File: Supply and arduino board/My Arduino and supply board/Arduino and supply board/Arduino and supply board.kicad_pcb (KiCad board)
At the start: 2 copper layers, 68.6 x 53.3 mm, 75 parts, among them IC1 MC33269ST-5.0T3-Arduino_and_s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, IC2 MC33269D-5.0-Arduino_and_supp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, Q1 16MHz, Q2 16MHz, T1 FDN340V, U1 LP2985-3.3, U1A1 LM358D, U1B1 LM358D, U1C1 LM358D, X1 USB_B, Y1 16MHz, Y2 16MHz

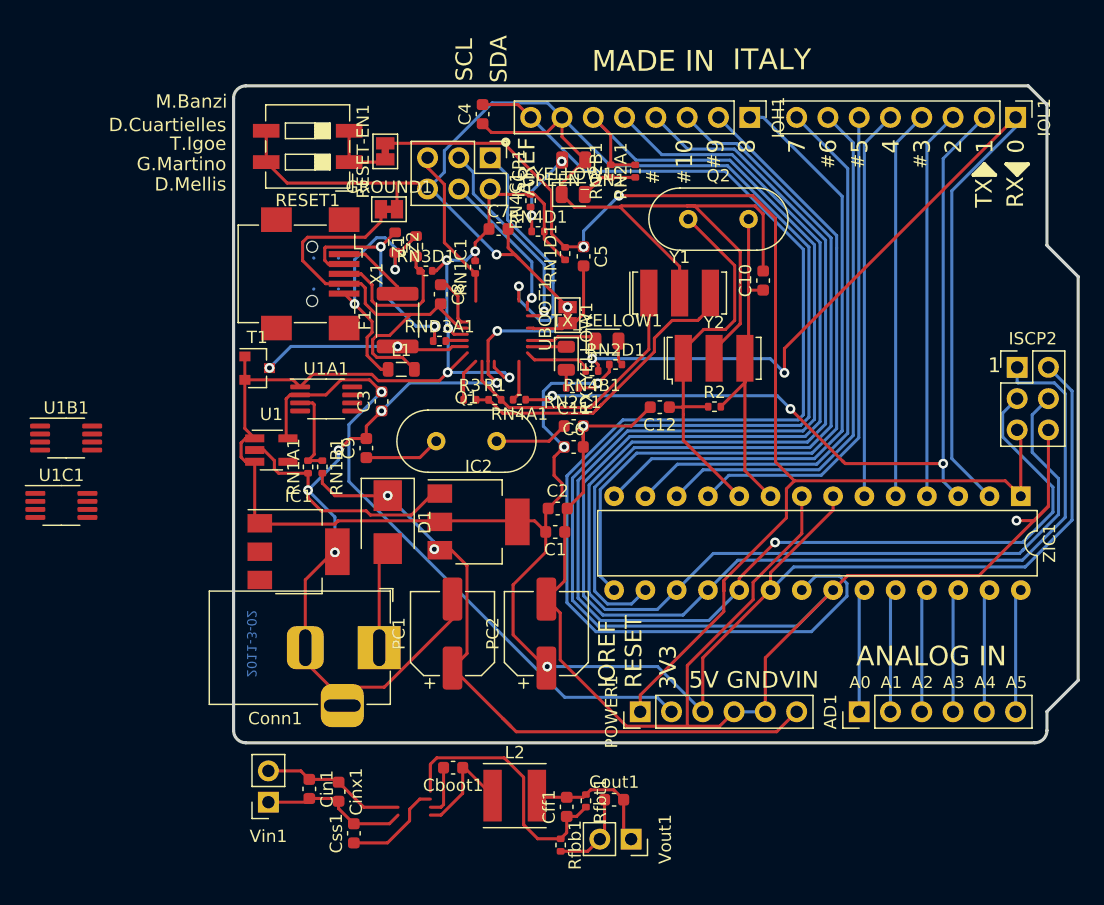
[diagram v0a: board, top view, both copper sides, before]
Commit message: new work on board
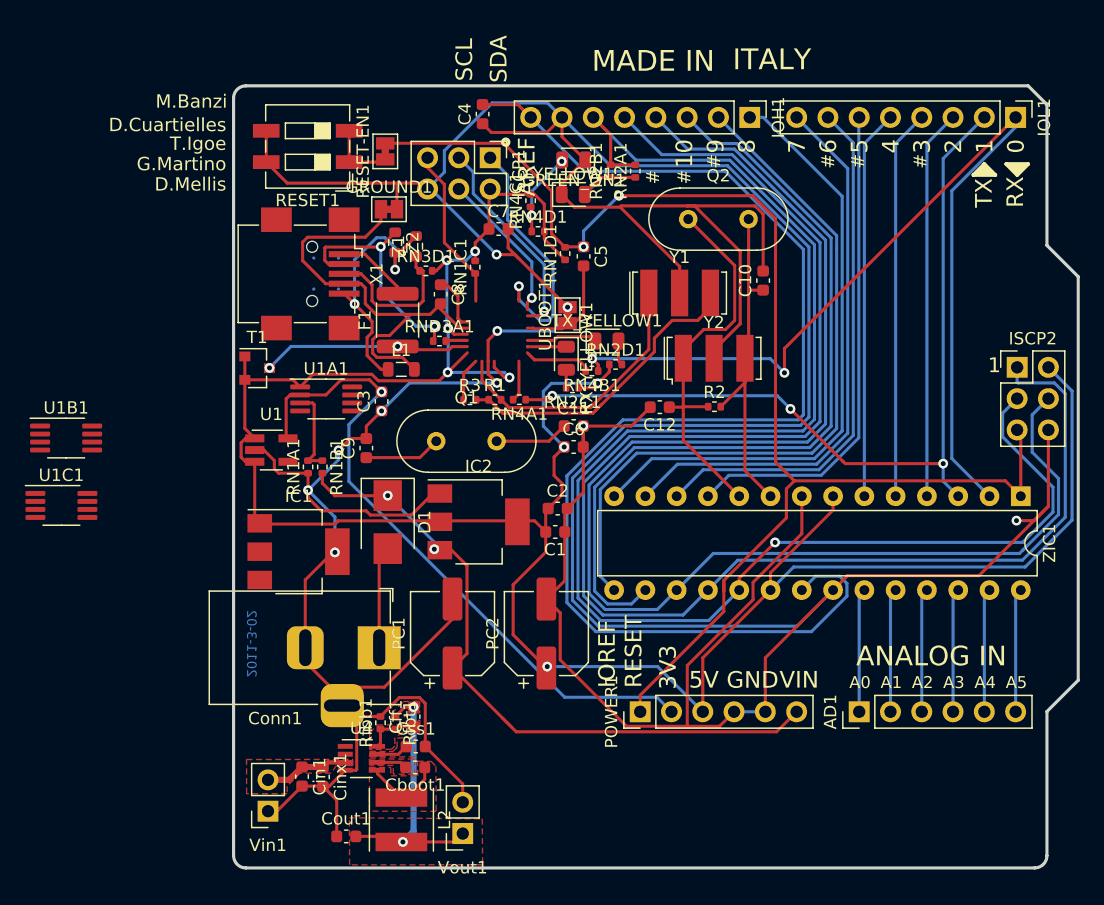
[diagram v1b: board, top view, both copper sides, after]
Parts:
- added U4: Arduino_and_supply_board-cache_Arduino_and_supply_board-cac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, Package_TO_SOT_SMD:TSOT-23-8, F.Cu at (142.6, 100.9)
- moved Cout1 22.0 mm to (141.4, 107.3)
- moved Rfbb1 17.7 mm to (144.1, 98.0), turned to 90 degrees
- moved Rfbt1 16.7 mm to (145.3, 98.1)
- moved Cff1 14.4 mm to (146.8, 97.6)
- moved Vout1 13.7 mm to (150.8, 107.0), turned to 180 degrees
- moved L2 9.41 mm to (145.8, 105.9), turned to 270 degrees
- moved Css1 8.65 mm to (147.0, 100.0), turned to 0 degrees
- moved Cboot1 3.08 mm to (147.0, 101.7)
- moved Cinx1 1.75 mm to (139.5, 102.4)
- moved Cin1 1.17 mm to (137.8, 102.4)
- moved Vin1 0.73 mm to (135.0, 105.2)
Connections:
- Cboot1 pad 2: (no net) -> Net-(Cboot1-Pad2)
- Css1 pad 1: (no net) -> Net-(Css1-Pad1)
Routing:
- net (no net): track 0.09 -> 77.8 mm, vias 0 -> 3
- net /MISO2: track 20.9 -> 0.00 mm, vias 1 -> 0
- net Net-(Cff1-Pad1): track 21.9 -> 4.30 mm
- net GND: track 421.3 -> 438.3 mm
- net /SCK2: track 16.9 -> 0.00 mm, vias 1 -> 0
- net /MOSI2: track 12.4 -> 0.00 mm, vias 1 -> 0
- net Net-(Cff1-Pad2): track 11.1 -> 22.3 mm, vias 0 -> 2
- net /TXLED: track 5.79 -> 0.00 mm
- net Net-(Css1-Pad1): track 8.23 -> 2.59 mm
- net /M8RXD: track 5.53 -> 0.00 mm
- net Net-(Cin1-Pad1): track 11.8 -> 6.88 mm
- net /VUCAP: track 4.48 -> 0.00 mm
- net Net-(R3-Pad1): track 3.54 -> 0.00 mm
- net /M8TXD: track 3.32 -> 0.00 mm
- net /RXLED: track 3.17 -> 0.00 mm
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- added copper zone on F.Cu, net Net-(Cboot1-Pad1)
- added copper zone on F.Cu, net Net-(Cboot1-Pad2)
- added copper zone on F.Cu, net Net-(Cff1-Pad1)
- added copper zone on F.Cu, net Net-(Cff1-Pad2)
- added copper zone on F.Cu, net Net-(Cin1-Pad1)
- added copper zone on F.Cu, net Net-(Css1-Pad1)
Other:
- board size 68.6 x 53.3 mm -> 68.6 x 63.5 mm
